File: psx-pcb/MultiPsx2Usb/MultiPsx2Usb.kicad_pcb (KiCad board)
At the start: 2 copper layers, 1 part

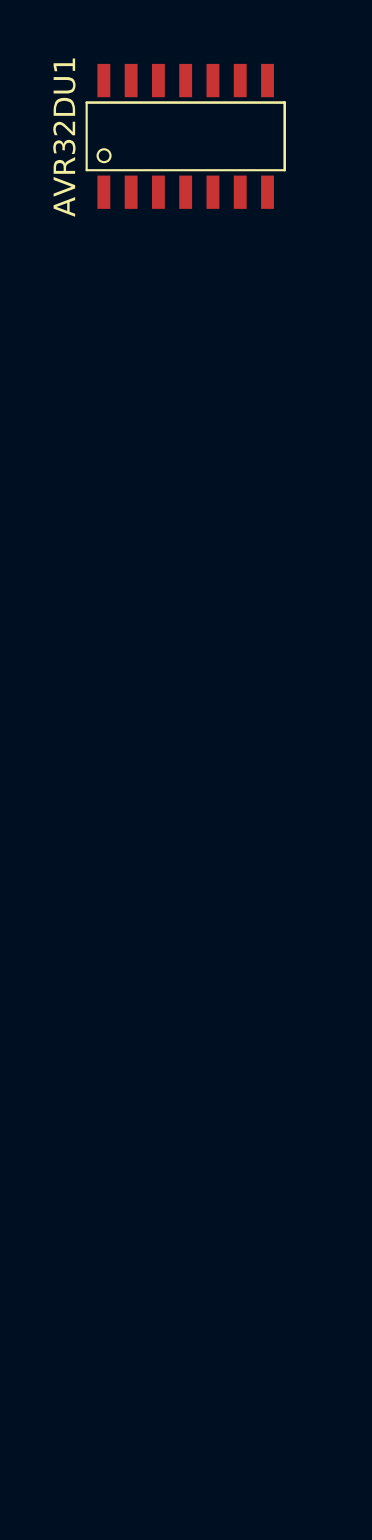
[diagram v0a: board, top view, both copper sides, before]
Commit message: Rough schematic mockup done. need to create test circuits and see what works and what doesn't.
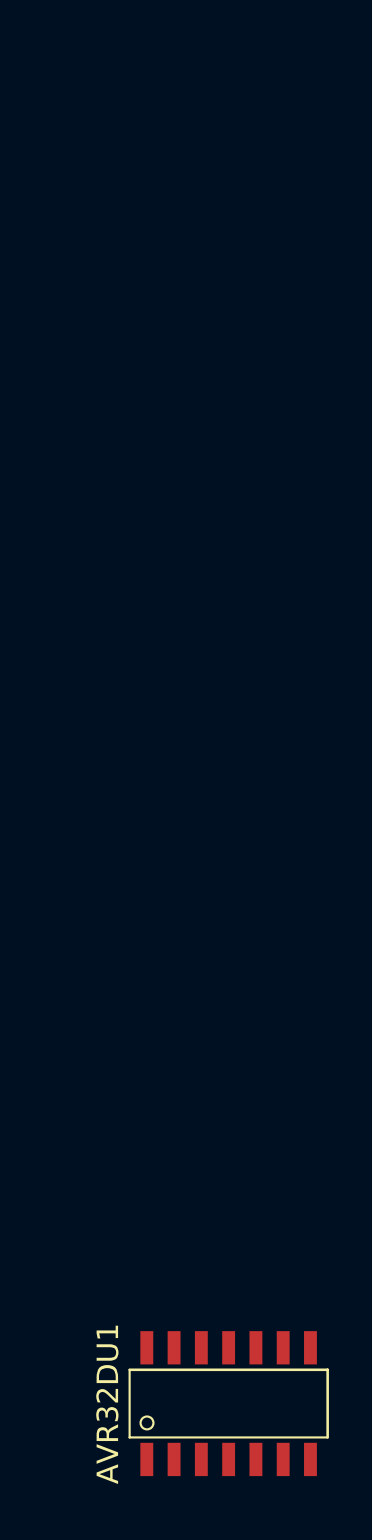
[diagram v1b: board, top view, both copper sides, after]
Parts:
- moved AVR32DU1 59.0 mm to (144.7, 148.1)
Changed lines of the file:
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@@
 	(footprint "avr32du:SOIC-14"
 		(layer "F.Cu")
-		(at 142.67 89.145)
+		(at 144.67 148.145)
 		(property "Reference" "AVR32DU1"
 			(at -5.61 0 90)
